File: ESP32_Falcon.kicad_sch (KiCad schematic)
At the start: 28 parts, among them J1 USB_C_Receptacle_USB2.0_16P, J2 Conn_01x20_Pin, J3 Conn_01x20_Pin, U1 ESP32-S3-WROOM-1, U2 USBLC6-2SC6, U3 AMS1117-3.3, U4 BMI270

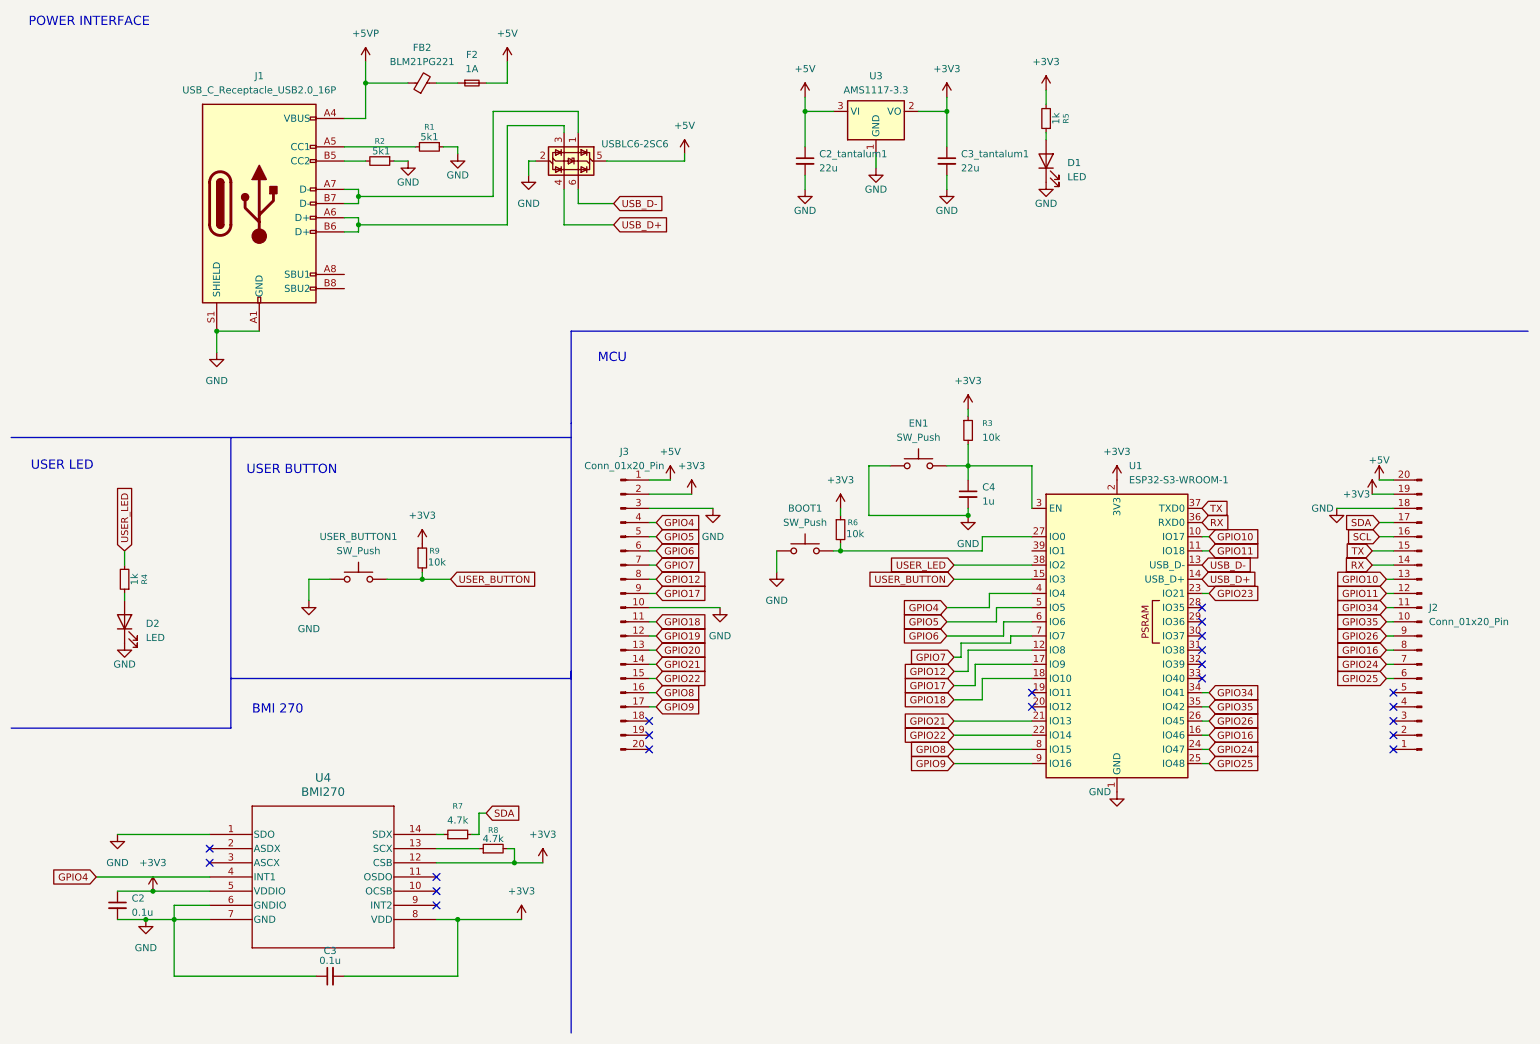
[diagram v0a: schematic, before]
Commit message: skończony projekt
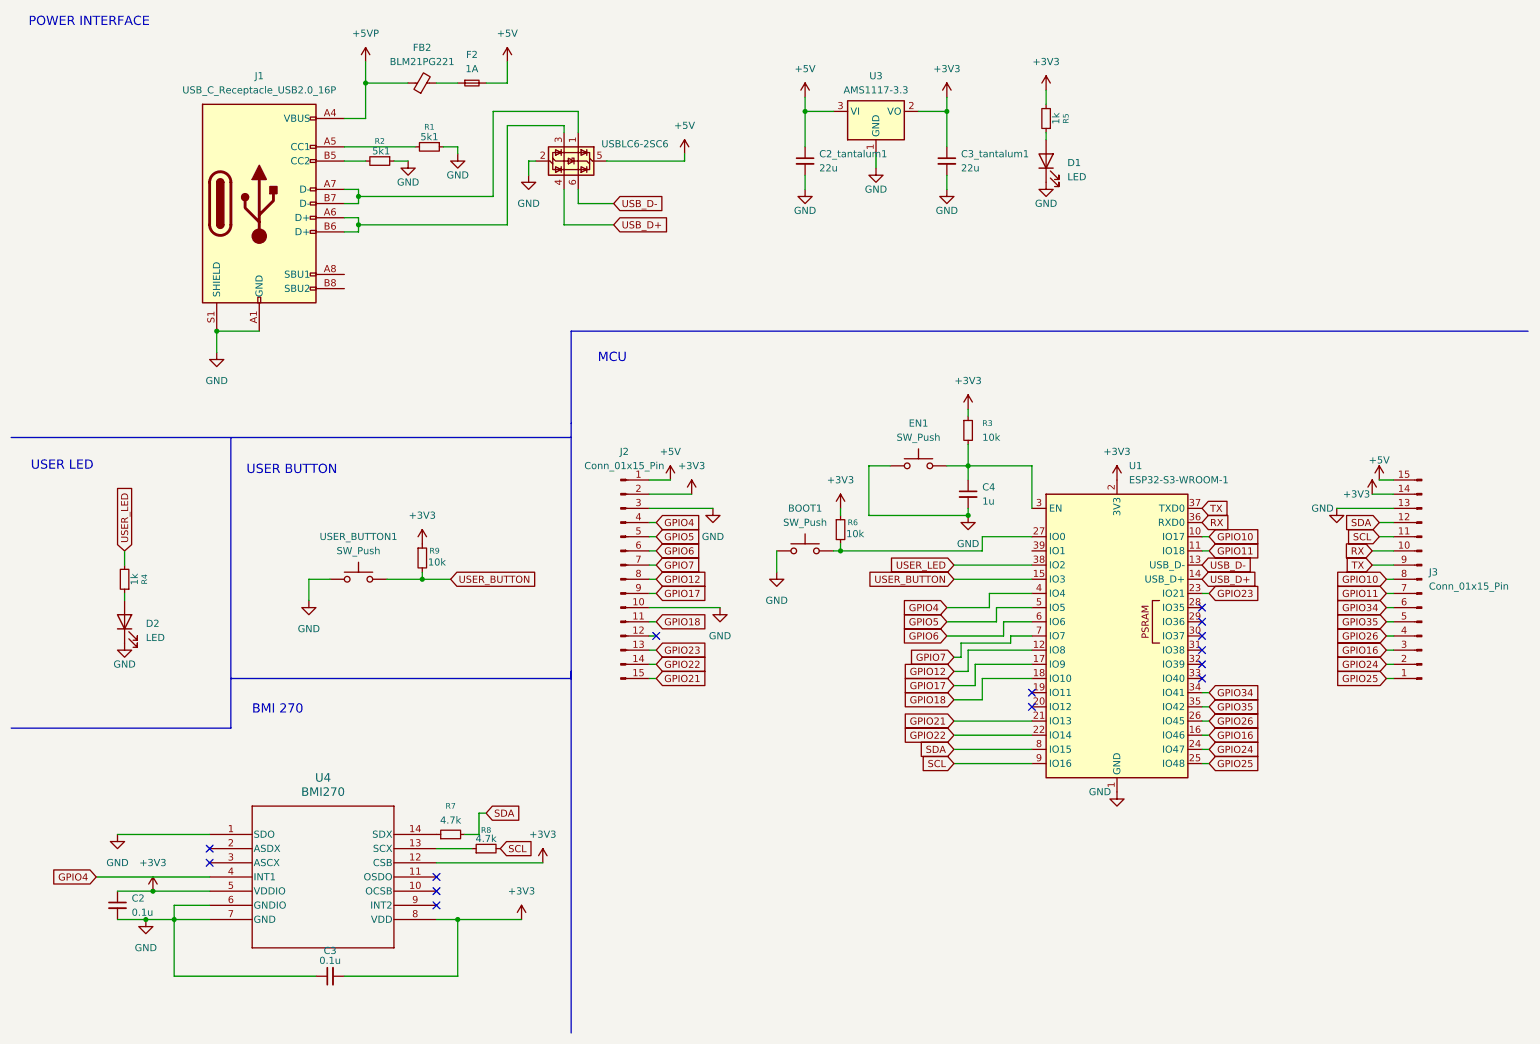
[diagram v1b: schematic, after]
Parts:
- removed J2, J3: Conn_01x20_Pin, Connector_PinHeader_2.54mm:PinHeader_1x20_P2.54mm_Vertical, symbol Connector:Conn_01x20_Pin
- added J2, J3: Conn_01x15_Pin, Connector_PinHeader_2.54mm:PinHeader_1x15_P2.54mm_Vertical, symbol Connector:Conn_01x15_Pin
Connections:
- net GPIO8 is gone; now on net SDA: U1.8 (IO15)
- net GPIO9 is gone; now on net SCL: U1.9 (IO16)
- net +3V3: now also J2.2 (Pin_2), J3.14 (Pin_14); no longer R8.2
- net +5V: now also J2.1 (Pin_1), J3.15 (Pin_15)
- net GND: now also J2.10 (Pin_10), J2.3 (Pin_3), J3.13 (Pin_13)
- net GPIO10: now also J3.8 (Pin_8)
- net GPIO11: now also J3.7 (Pin_7)
- net GPIO12: now also J2.8 (Pin_8)
- net GPIO16: now also J3.3 (Pin_3)
- net GPIO17: now also J2.9 (Pin_9)
- net GPIO18: now also J2.11 (Pin_11)
- net GPIO21: now also J2.15 (Pin_15)
- net GPIO22: now also J2.14 (Pin_14)
- net GPIO23: now also J2.13 (Pin_13)
- net GPIO24: now also J3.2 (Pin_2)
- net GPIO25: now also J3.1 (Pin_1)
- net GPIO26: now also J3.4 (Pin_4)
- net GPIO34: now also J3.6 (Pin_6)
- net GPIO35: now also J3.5 (Pin_5)
- net GPIO4: now also J2.4 (Pin_4)
- net GPIO5: now also J2.5 (Pin_5)
- net GPIO6: now also J2.6 (Pin_6)
- net GPIO7: now also J2.7 (Pin_7)
- net RX: now also J3.10 (Pin_10)
- net SCL: now also R8.2, J3.11 (Pin_11)
- net SDA: now also J3.12 (Pin_12)
- net TX: now also J3.9 (Pin_9)
- no-connect marks 21 -> 14
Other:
- moved on the sheet: R7, R8
